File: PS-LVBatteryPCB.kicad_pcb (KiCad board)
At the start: 2 copper layers, 28.3 x 31.8 mm, 10 parts, among them J1 NTC_01, J2 NTC_02, J3 NTC_OUT, J4 SUPP+, J5 SUPP_GND, J6 SUPP_FUSE

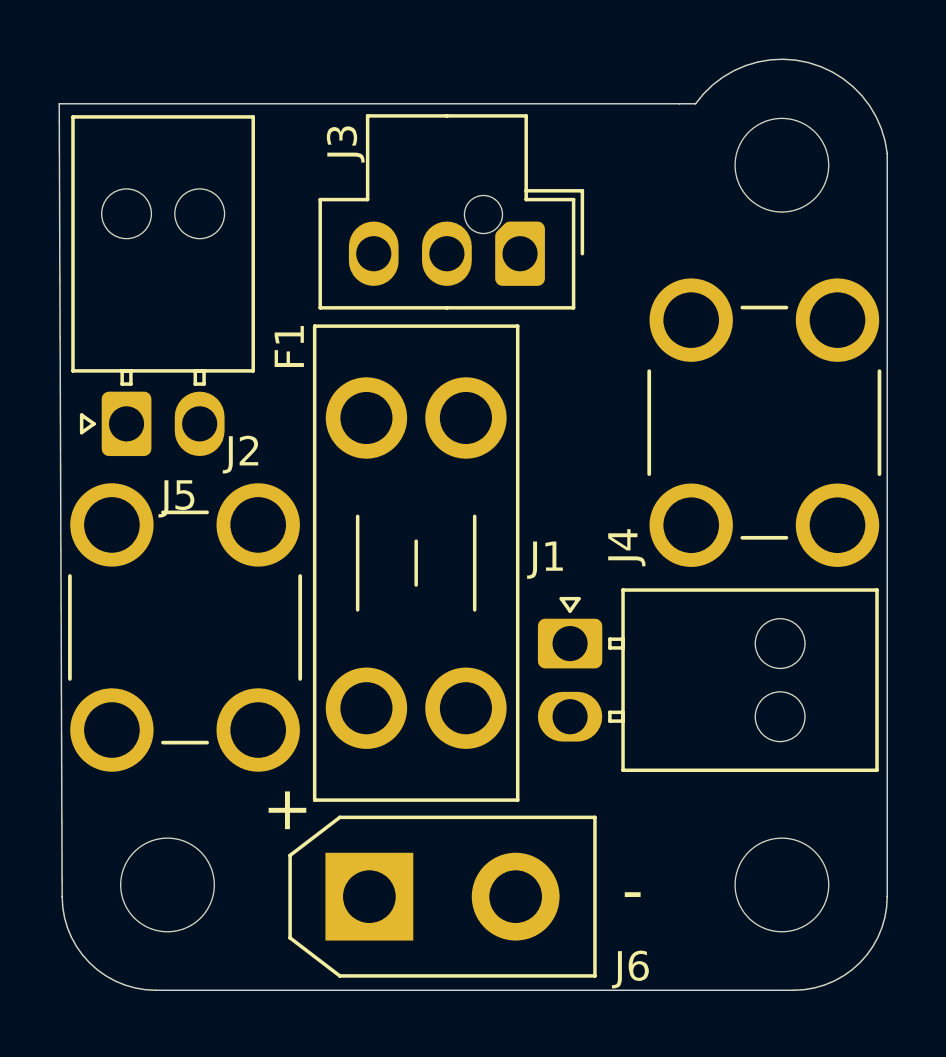
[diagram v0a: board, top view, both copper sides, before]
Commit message: R1
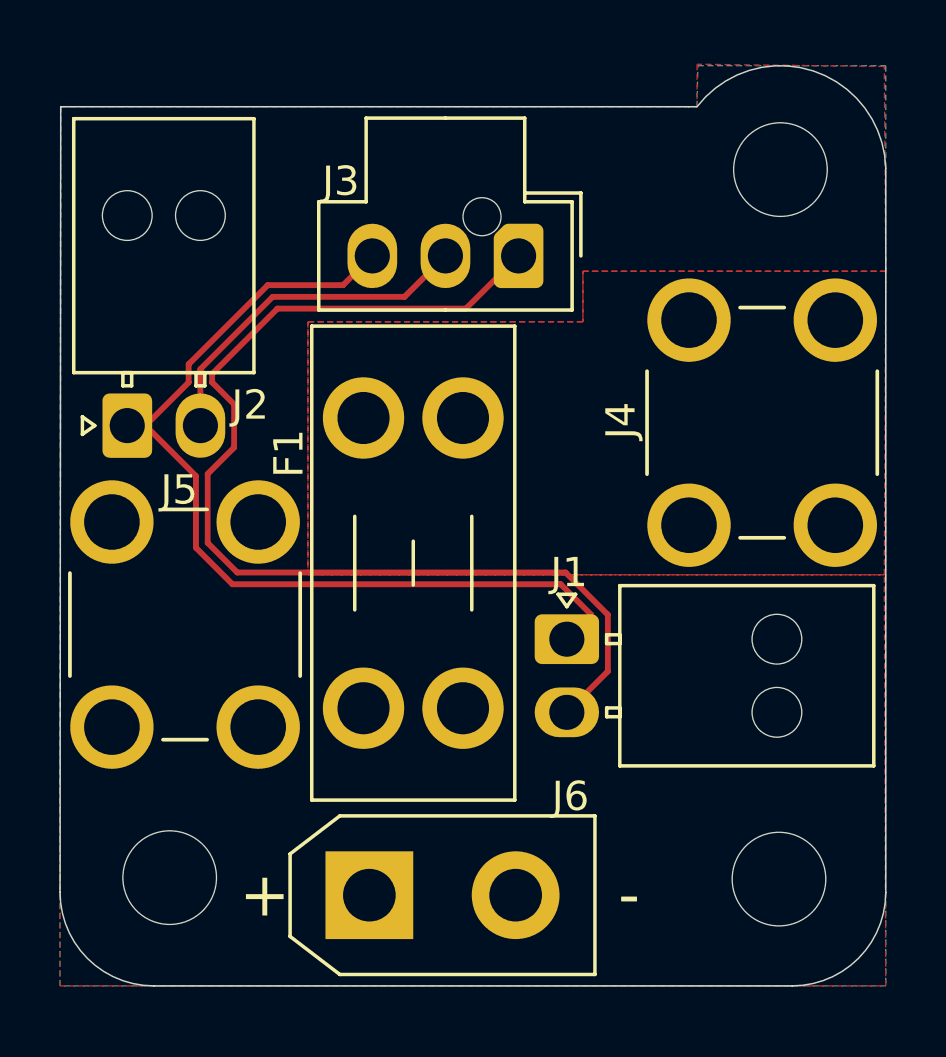
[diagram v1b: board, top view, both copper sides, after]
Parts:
- moved REF** 0.26 mm to (130.7, 113.0)
- moved REF** 0.22 mm to (151.5, 113.0)
- moved J1 0.19 mm to (144.2, 104.8)
- moved REF** 0.16 mm to (151.6, 88.8)
- moved F1 0.10 mm to (140.7, 97.2)
- moved J5 0.10 mm to (131.2, 104.3)
- moved J3 0.09 mm to (142.6, 91.7)
- moved J4 0.07 mm to (150.9, 97.4)
- moved J2 0.07 mm to (129.2, 97.5)
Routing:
- net Net-(J1-Pin_2): track 0.00 -> 37.2 mm
- net Net-(J1-Pin_1): track 0.00 -> 31.7 mm
- net Net-(J2-Pin_2): track 0.00 -> 11.9 mm
- added copper zone on F.Cu, net /SUPP+
- added copper zone on F.Cu, net /SUPP_FUSE+
- added copper zone on B.Cu, net /SUPP_GND
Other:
- board size 28.3 x 31.8 mm -> 28.2 x 31.4 mm
